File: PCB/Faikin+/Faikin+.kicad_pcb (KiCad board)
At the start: 2 copper layers, 70 x 70 mm, 32 parts, among them J1 1x5, J2 Shelly, J3 USB-PROG, J4 1x5, Q1 BSS138PS, Q2 BSS138PS, U3 MD8942, U4 ESP32-S3-MINI-1

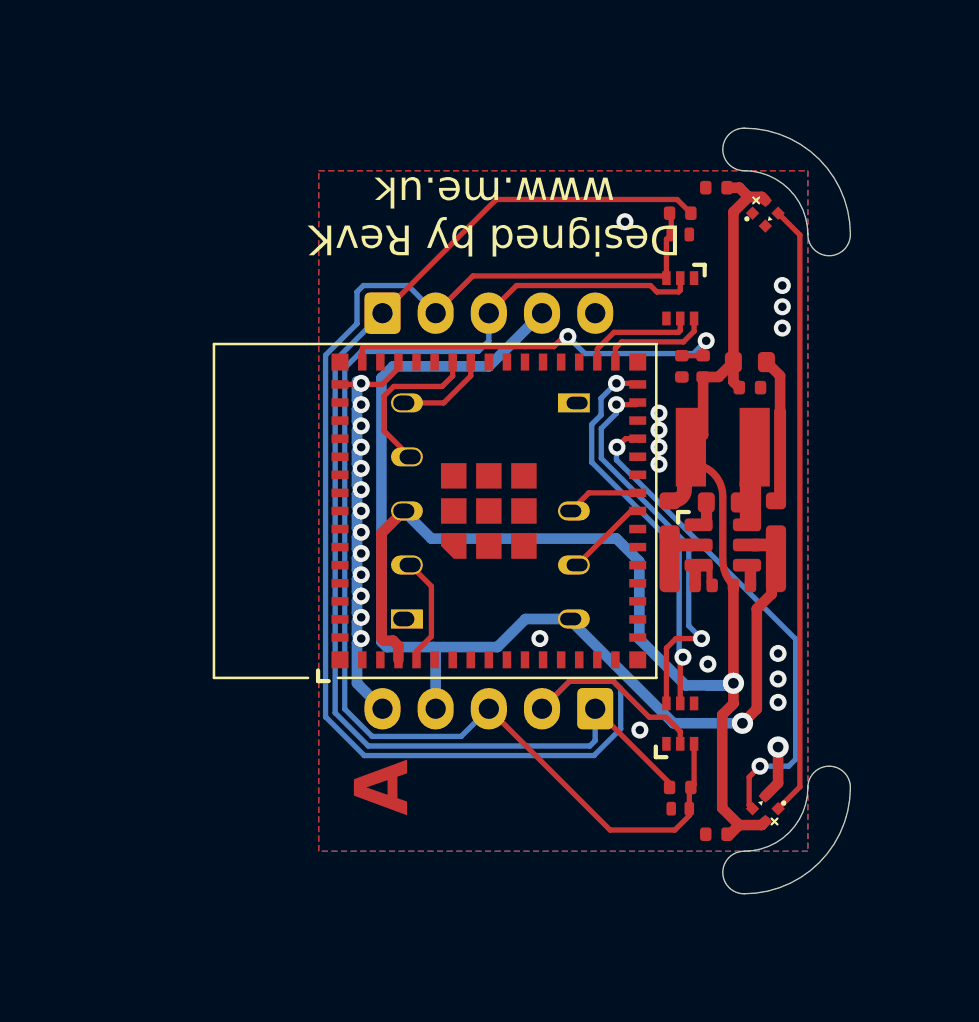
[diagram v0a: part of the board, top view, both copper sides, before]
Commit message: New board
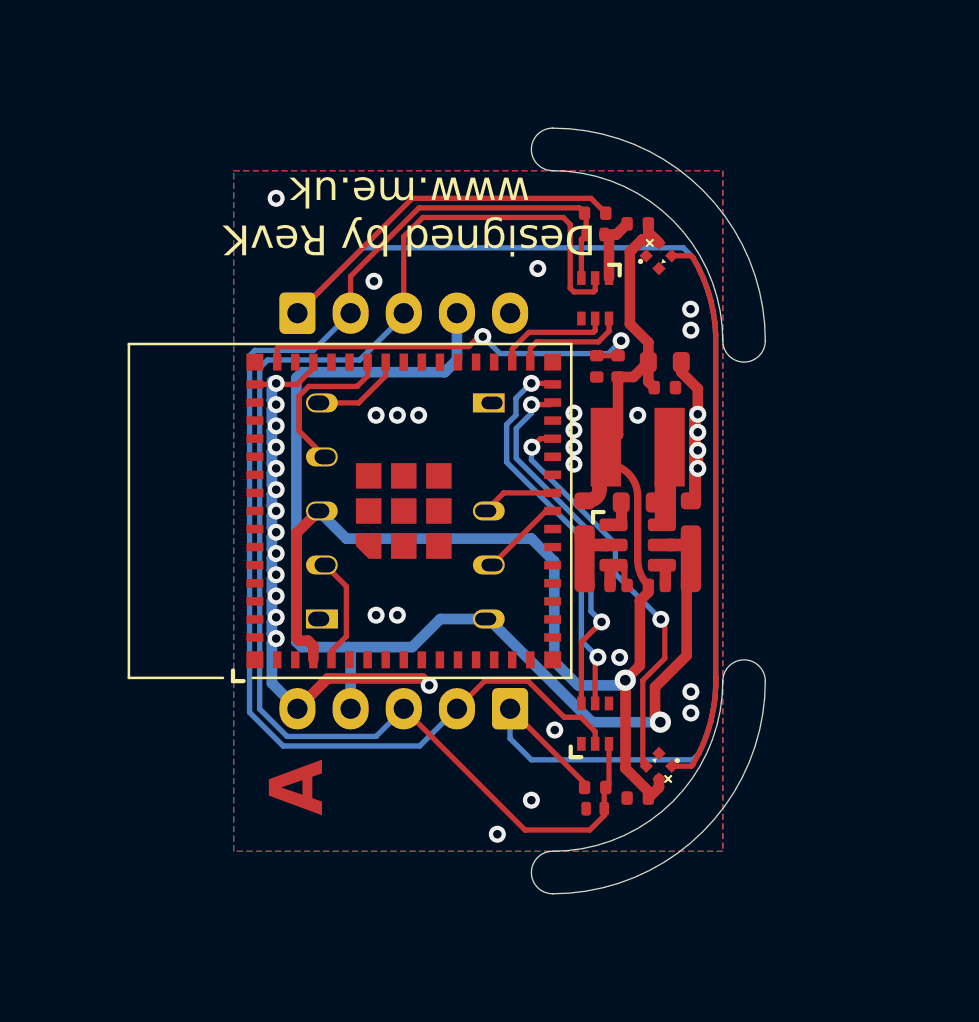
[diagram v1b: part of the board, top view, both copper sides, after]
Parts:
- moved D1 5.39 mm to (143.0, 76.0)
- moved D4 5.39 mm to (143.0, 52.0)
- moved C1 4.07 mm to (142.0, 50.5)
- moved C3 4.07 mm to (142.0, 77.5)
- moved C10 4.00 mm to (142.0, 63.6)
- moved C2 4.00 mm to (143.3, 58.2)
- moved C5 4.00 mm to (143.3, 57.0)
- moved C6 4.00 mm to (140.1, 57.2)
- moved C8 4.00 mm to (144.5, 64.3)
- moved C9 4.00 mm to (139.5, 64.3)
- moved D2 4.00 mm to (140.0, 78.0)
- moved D3 4.00 mm to (140.0, 51.0)
- moved J1 4.00 mm to (136.0, 73.3)
- moved J2 4.00 mm to (127.2, 64.0)
- moved J3 4.00 mm to (135.0, 64.0)
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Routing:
- net Net-(J1-Pin_1): track 56.3 -> 76.7 mm
- net S21RX: track 69.8 -> 59.3 mm
- net GND: track 28.5 -> 36.2 mm, vias 28 -> 39
- net S21TX: track 58.3 -> 63.9 mm
- net +3.3V: track 60.8 -> 55.6 mm
- net LED: track 23.4 -> 19.2 mm
- net Net-(D1-O): track 28.8 -> 26.3 mm
- net RX: track 18.7 -> 17.4 mm
- net DC: track 51.5 -> 52.2 mm

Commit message: 4 vcuts
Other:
- board text added: "4 V-cuts"
- board text removed: "6 V-cuts"
